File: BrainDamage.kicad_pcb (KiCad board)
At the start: 2 copper layers, 90 x 90 mm, 25 parts, among them CON1 AVR-ISP-10, IC1 ATMEGA328P-A, P1 CONN_01X03, P10 CONN_01X03, P11 CONN_01X03, P12 CONN_01X03, P13 CONN_01X03, P14 CONN_01X03, P15 CONN_01X03, P16 CONN_01X03, P17 CONN_01X03, P2 CONN_01X03, P3 CONN_01X03, P4 CONN_01X03, P5 CONN_01X03, P6 CONN_01X03, P7 CONN_01X03, P8 CONN_01X08, P9 CONN_01X03, SW1 SW_PUSH, U1 PCA9685-TSSOP

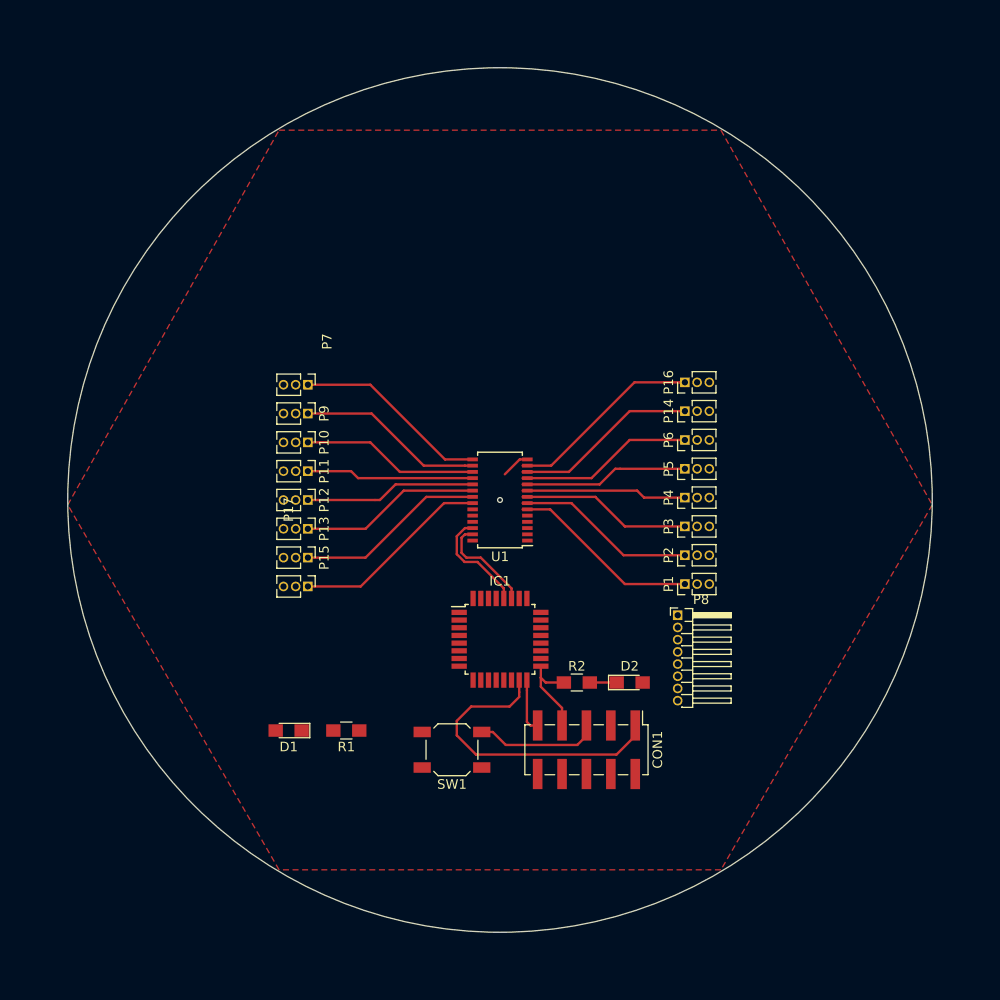
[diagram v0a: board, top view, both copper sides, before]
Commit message: Add files via upload
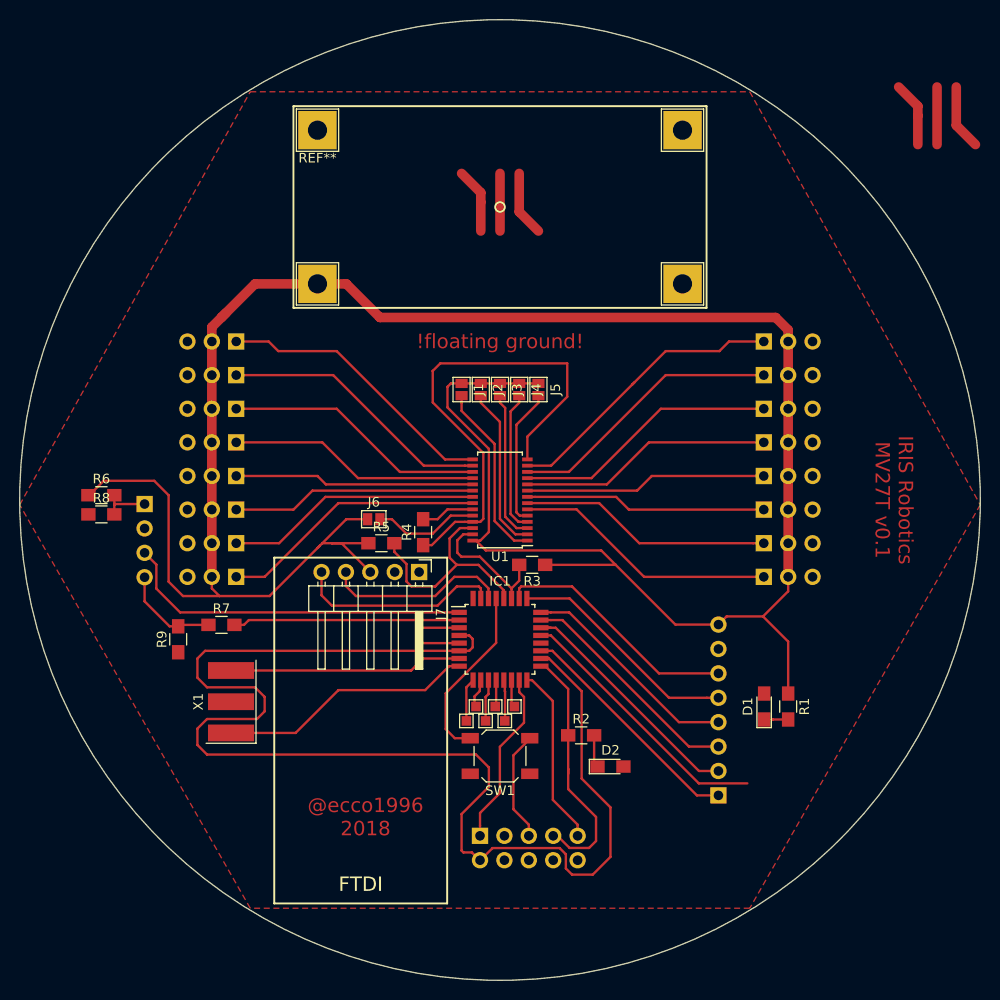
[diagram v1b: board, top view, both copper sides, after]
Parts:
- added J1: TEST_2P, Connectors:GS2, F.Cu at (196.0, 52.0)
- added J2: TEST_2P, Connectors:GS2, F.Cu at (198.0, 52.0)
- added J3: TEST_2P, Connectors:GS2, F.Cu at (200.0, 52.0)
- added J4: TEST_2P, Connectors:GS2, F.Cu at (202.0, 52.0)
- added J5: TEST_2P, Connectors:GS2, F.Cu at (204.0, 52.0)
- added J6: TEST_2P, Connectors:GS2, F.Cu at (186.9, 65.5)
- added J7: FTDI, Pin_Headers:Pin_Header_Angled_1x05_Pitch2.54mm, F.Cu at (191.6, 71.0)
- added J8: Bluetooth, Pin_Headers:Pin_Header_Straight_1x04_Pitch2.54mm, B.Cu at (163.0, 63.9)
- added R3: 10K, Resistors_SMD:R_0805_HandSoldering, F.Cu at (203.3, 70.2)
- added R4: 10K, Resistors_SMD:R_0805_HandSoldering, F.Cu at (192.0, 66.8)
- added R5: 10K, Resistors_SMD:R_0805_HandSoldering, F.Cu at (187.7, 68.0)
- added R6: 20K, Resistors_SMD:R_0805_HandSoldering, F.Cu at (158.5, 63.0)
- added R7: 20K, Resistors_SMD:R_0805_HandSoldering, F.Cu at (171.0, 76.5)
- added R8: 10K, Resistors_SMD:R_0805_HandSoldering, F.Cu at (158.5, 65.0)
- added R9: 10K, Resistors_SMD:R_0805_HandSoldering, F.Cu at (166.5, 78.0)
- added REF**: Test_Point_Pad_1.0x1.0mm, Connectors_TestPoints:Test_Point_Pad_1.0x1.0mm, F.Cu at (200.5, 86.5)
- added REF**: Test_Point_THTPad_4.0x4.0mm_Drill2.0mm, Connectors_TestPoints:Test_Point_THTPad_4.0x4.0mm_Drill2.0mm, F.Cu at (219.0, 25.0)
- added REF**: Test_Point_Pad_1.0x1.0mm, Connectors_TestPoints:Test_Point_Pad_1.0x1.0mm, F.Cu at (199.5, 85.0)
- added REF**: Test_Point_Pad_1.0x1.0mm, Connectors_TestPoints:Test_Point_Pad_1.0x1.0mm, F.Cu at (198.5, 86.5)
- added REF**: Test_Point_Pad_1.0x1.0mm, Connectors_TestPoints:Test_Point_Pad_1.0x1.0mm, F.Cu at (197.5, 85.0)
- added REF**: Test_Point_Pad_1.0x1.0mm, Connectors_TestPoints:Test_Point_Pad_1.0x1.0mm, F.Cu at (201.5, 85.0)
- added REF**: Test_Point_Pad_1.0x1.0mm, Connectors_TestPoints:Test_Point_Pad_1.0x1.0mm, F.Cu at (196.5, 86.5)
- added REF**: Test_Point_THTPad_4.0x4.0mm_Drill2.0mm, Connectors_TestPoints:Test_Point_THTPad_4.0x4.0mm_Drill2.0mm, F.Cu at (181.0, 25.0)
- added REF**: Test_Point_THTPad_4.0x4.0mm_Drill2.0mm, Connectors_TestPoints:Test_Point_THTPad_4.0x4.0mm_Drill2.0mm, F.Cu at (181.0, 41.0)
- added REF**: Test_Point_THTPad_4.0x4.0mm_Drill2.0mm, Connectors_TestPoints:Test_Point_THTPad_4.0x4.0mm_Drill2.0mm, F.Cu at (219.0, 41.0)
- added X1: CRYSTAL_SMD, Crystals:Resonator_SMD_muRata_SFSKA-3pin_7.9x3.8mm_HandSoldering, F.Cu at (172.0, 84.5)
- CON1: footprint Pin_Headers:Pin_Header_Straight_2x05_Pitch2.54mm_SMD -> Pin_Headers:Pin_Header_Straight_2x05_Pitch2.54mm; moved to B.Cu
- P1, P10, P11, P12, P13, P14, P15, P16, P17, P2, P3, P4, P5, P6, P7, P9: footprint Pin_Headers:Pin_Header_Straight_1x03_Pitch1.27mm -> Pin_Headers:Pin_Header_Straight_1x03_Pitch2.54mm; moved to B.Cu
- P8: footprint Pin_Headers:Pin_Header_Angled_1x08_Pitch1.27mm -> Pin_Headers:Pin_Header_Angled_1x08_Pitch2.54mm; moved to B.Cu
- moved D1 49.6 mm to (227.5, 85.0), turned to 90 degrees
- moved R1 46.1 mm to (230.0, 85.0), turned to 270 degrees
- moved P17 26.6 mm to (172.5, 47.0), turned to 90 degrees
- moved P1 26.6 mm to (227.5, 47.0), turned to 270 degrees
- moved P16 21.9 mm to (227.5, 71.5), turned to 270 degrees
- moved P7 21.3 mm to (172.5, 71.5), turned to 90 degrees
- moved P2 20.5 mm to (227.5, 50.5), turned to 270 degrees
- moved P15 20.4 mm to (172.5, 50.5), turned to 90 degrees
- moved P8 19.2 mm to (222.7, 94.2)
- moved P14 16.0 mm to (227.5, 68.0), turned to 270 degrees
- moved P9 15.4 mm to (172.5, 68.0), turned to 90 degrees
- moved P3 14.7 mm to (227.5, 54.0), turned to 270 degrees
- moved P13 14.6 mm to (172.5, 54.0), turned to 90 degrees
- moved CON1 14.2 mm to (197.9, 98.5)
- moved P6 11.0 mm to (227.5, 64.5), turned to 270 degrees
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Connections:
- net Net-(IC1-Pad32) renamed /PD2
- CON1 pad 2: +3V3 -> +5V
- IC1 pad 1: /PIN6 -> /TXB
- IC1 pad 10: /PIN4 -> /PD6
- IC1 pad 11: Net-(IC1-Pad11) -> /PD7
- IC1 pad 12: /B1 -> /PB0
- IC1 pad 13: /PIN1 -> /PB1
- IC1 pad 14: /PIN2 -> /PB2
- IC1 pad 2: Net-(IC1-Pad2) -> /RXB
- IC1 pad 23: /A0 -> /PC0
- IC1 pad 24: /A1 -> /PC1
- IC1 pad 25: /A2 -> /PC2
- IC1 pad 26: /A3 -> /PC3
- IC1 pad 9: /PIN5 -> /PD5
- P1 pad 1: /LED0 -> /LED7
- P1 pad 2: +3V3 -> +5V
- P10 pad 1: /LED10 -> /LED13
- P10 pad 2: +3V3 -> +5V
- P11 pad 1: /LED11 -> /LED12
- P11 pad 2: +3V3 -> +5V
- P12 pad 1: /LED12 -> /LED11
- P12 pad 2: +3V3 -> +5V
- P13 pad 1: /LED13 -> /LED10
- P13 pad 2: Net-(P13-Pad2) -> +5V
- P14 pad 1: /LED6 -> /LED1
- P14 pad 2: +3V3 -> +5V
- P15 pad 1: /LED14 -> /LED9
- P15 pad 2: +3V3 -> +5V
- P16 pad 1: /LED7 -> /LED0
- P16 pad 2: +3V3 -> +5V
- P17 pad 1: /LED15 -> /LED8
- P17 pad 2: +3V3 -> +5V
- P2 pad 1: /LED1 -> /LED6
- P2 pad 2: +3V3 -> +5V
- P3 pad 1: /LED2 -> /LED5
- P3 pad 2: +3V3 -> +5V
- P4 pad 1: /LED3 -> /LED4
- P4 pad 2: +3V3 -> +5V
- P5 pad 1: /LED4 -> /LED3
- P5 pad 2: +3V3 -> +5V
- P6 pad 1: /LED5 -> /LED2
- P6 pad 2: Net-(P6-Pad2) -> +5V
- P7 pad 1: /LED8 -> /LED15
- P7 pad 2: +3V3 -> +5V
- P8 pad 1: /SCL -> /ADC6
- P8 pad 2: /SDA -> /ADC7
- P8 pad 3: /A3 -> /PC0
- P8 pad 4: /A2 -> /PC1
- P8 pad 5: /A1 -> /PC2
- P8 pad 6: /A0 -> /PC3
- P8 pad 7: /ADC7 -> GND
- P8 pad 8: /ADC6 -> +5V
- P9 pad 1: /LED9 -> /LED14
- P9 pad 2: +3V3 -> +5V
- U1 pad 1: Net-(U1-Pad1) -> /A0
- U1 pad 2: Net-(U1-Pad2) -> /A1
- U1 pad 23: Net-(U1-Pad23) -> /OE
- U1 pad 24: Net-(U1-Pad24) -> /A5
- U1 pad 25: Net-(U1-Pad25) -> GND
- U1 pad 3: Net-(U1-Pad3) -> /A2
- U1 pad 4: Net-(U1-Pad4) -> /A3
- U1 pad 5: Net-(U1-Pad5) -> /A4
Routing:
- net +5V: track 0.00 -> 394.2 mm
- net GND: track 2.99 -> 89.5 mm
- net (no net): track 0.00 -> 39.3 mm
- net /TXB: track 0.00 -> 36.8 mm
- net /ADC7: track 0.00 -> 26.3 mm
- net /PC3: track 0.00 -> 25.6 mm
- net /XTAL2: track 0.00 -> 24.9 mm
- net /ADC6: track 0.00 -> 24.7 mm
- net /PC2: track 0.00 -> 24.2 mm
- net /PC0: track 0.00 -> 23.9 mm
- net /RXB: track 0.00 -> 23.6 mm
- net /PC1: track 0.00 -> 23.2 mm
- net /XTAL1: track 0.00 -> 22.4 mm
- net /TX: track 0.00 -> 21.4 mm
- net /RX: track 0.00 -> 19.1 mm
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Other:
- board size 90 x 90 mm -> 100 x 100 mm
- net class Default: clearance 0.2 -> 0.25
- rule trace_clearance: 0.2 -> 0.25
- board text added: "!floating ground!"
- board text added: "@ecco1996 2018"
- board text added: "FTDI"
- board text added: "IRIS Robotics MV27T v0.1"
